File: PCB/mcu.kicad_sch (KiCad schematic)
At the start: 37 parts, among them J10 Conn_01x02, SW3 Reset, SW4 Boot, U1 LSM6DS3, U7 ESP32-S3, Y2 40MHz

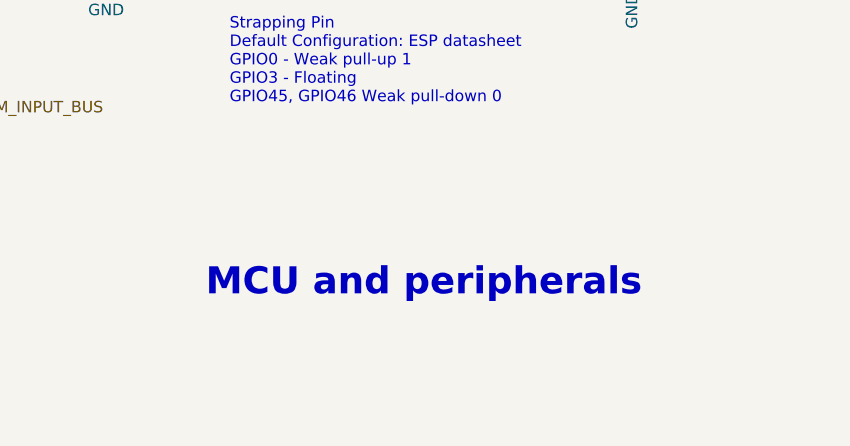
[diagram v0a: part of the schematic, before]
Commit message: Updates to README
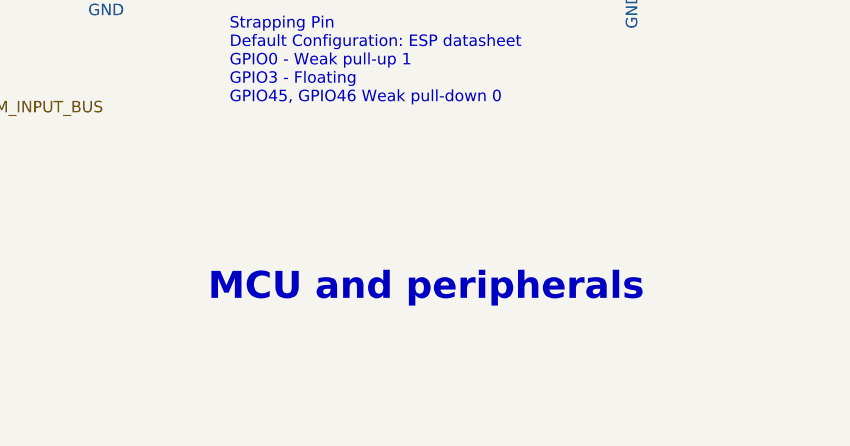
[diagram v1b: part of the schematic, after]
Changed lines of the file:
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@@
 	(text "MCU and peripherals"
 		(exclude_from_sim no)
-		(at 204.216 174.498 0)
+		(at 204.47 175.006 0)
 		(effects
 			(font
@@
 	(label "IO40"
 		(at 132.715 91.44 180)
-		(fields_autoplaced yes)
 		(effects
 			(font
@@
 	(label "IN[1..4]"
 		(at 137.16 154.94 0)
-		(fields_autoplaced yes)
 		(effects
 			(font
@@
 	(label "SDO"
 		(at 213.36 99.06 0)
-		(fields_autoplaced yes)
 		(effects
 			(font
@@
 	(label "IN1"
 		(at 125.73 147.32 180)
-		(fields_autoplaced yes)
 		(effects
 			(font
@@
 	(label "RX"
 		(at 217.17 60.96 0)
-		(fields_autoplaced yes)
 		(effects
 			(font
@@
 	(label "SDO"
 		(at 30.48 154.94 180)
-		(fields_autoplaced yes)
 		(effects
 			(font
@@
 	(label "SDA"
 		(at 213.36 101.6 0)
-		(fields_autoplaced yes)
 		(effects
 			(font
@@
 	(label "IN3"
 		(at 125.73 129.54 180)
-		(fields_autoplaced yes)
 		(effects
 			(font
@@
 	(label "CS"
 		(at 213.36 106.68 0)
-		(fields_autoplaced yes)
 		(effects
 			(font
@@
 	(label "IN2"
 		(at 125.73 119.38 180)
-		(fields_autoplaced yes)
 		(effects
 			(font
@@
 	(label "IN2"
 		(at 125.73 149.86 180)
-		(fields_autoplaced yes)
 		(effects
 			(font
@@
 	(label "SCL"
 		(at 213.36 104.14 0)
-		(fields_autoplaced yes)
 		(effects
 			(font
@@
 	(label "IO15"
 		(at 132.08 71.12 180)
-		(fields_autoplaced yes)
 		(effects
 			(font
@@
 	(label "IO41"
 		(at 132.715 93.98 180)
-		(fields_autoplaced yes)
 		(effects
 			(font
@@
 	(label "INT1"
 		(at 72.39 154.94 0)
-		(fields_autoplaced yes)
 		(effects
 			(font
@@
 	(label "IN4"
 		(at 125.73 152.4 180)
-		(fields_autoplaced yes)
 		(effects
 			(font
@@
 	(label "INT2"
 		(at 213.36 109.22 0)
-		(fields_autoplaced yes)
 		(effects
 			(font
@@
 	(label "INT1"
 		(at 212.725 96.52 0)
-		(fields_autoplaced yes)
 		(effects
 			(font
@@
 	(label "CS"
 		(at 25.4 170.18 180)
-		(fields_autoplaced yes)
 		(effects
 			(font
@@
 	(label "IO45"
 		(at 250.825 121.92 0)
-		(fields_autoplaced yes)
 		(effects
 			(font
@@
 	(label "IN1"
 		(at 125.73 121.92 180)
-		(fields_autoplaced yes)
 		(effects
 			(font
@@
 	(label "TX"
 		(at 217.17 58.42 0)
-		(fields_autoplaced yes)
 		(effects
 			(font
@@
 	(label "INT2"
 		(at 72.39 157.48 0)
-		(fields_autoplaced yes)
 		(effects
 			(font
@@
 	(label "IN4"
 		(at 125.73 127 180)
-		(fields_autoplaced yes)
 		(effects
 			(font
@@
 	(label "SDA"
 		(at 34.29 165.1 180)
-		(fields_autoplaced yes)
 		(effects
 			(font
@@
 	(label "IO42"
 		(at 132.715 96.52 180)
-		(fields_autoplaced yes)
 		(effects
 			(font
@@
 	(label "SCL"
 		(at 29.21 167.64 180)
-		(fields_autoplaced yes)
 		(effects
 			(font
@@
 	(label "IO16"
 		(at 132.08 73.66 180)
-		(fields_autoplaced yes)
 		(effects
 			(font
@@
 	(label "IN3"
 		(at 125.73 154.94 180)
-		(fields_autoplaced yes)
 		(effects
 			(font
@@
 		(shape output)
 		(at 154.94 154.94 0)
-		(fields_autoplaced yes)
 		(effects
 			(font
@@
 		(shape input)
 		(at 213.36 114.3 0)
-		(fields_autoplaced yes)
 		(effects
 			(font
@@
 		(shape bidirectional)
 		(at 214.63 66.04 0)
-		(fields_autoplaced yes)
 		(effects
 			(font
@@
 		(shape bidirectional)
 		(at 214.63 68.58 0)
-		(fields_autoplaced yes)
 		(effects
 			(font
@@
 		(shape input)
 		(at 219.71 93.98 0)
-		(fields_autoplaced yes)
 		(effects
 			(font
@@
 		(shape output)
 		(at 121.92 124.46 180)
-		(fields_autoplaced yes)
 		(effects
 			(font
@@
 		(shape input)
 		(at 218.44 119.38 0)
-		(fields_autoplaced yes)
-		(effects
-			(font
+		(effects
+			(font
